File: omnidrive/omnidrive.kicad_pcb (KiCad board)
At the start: 2 copper layers, 76.2 x 27.9 mm, 73 parts, among them U1 TL072, U2 TL072

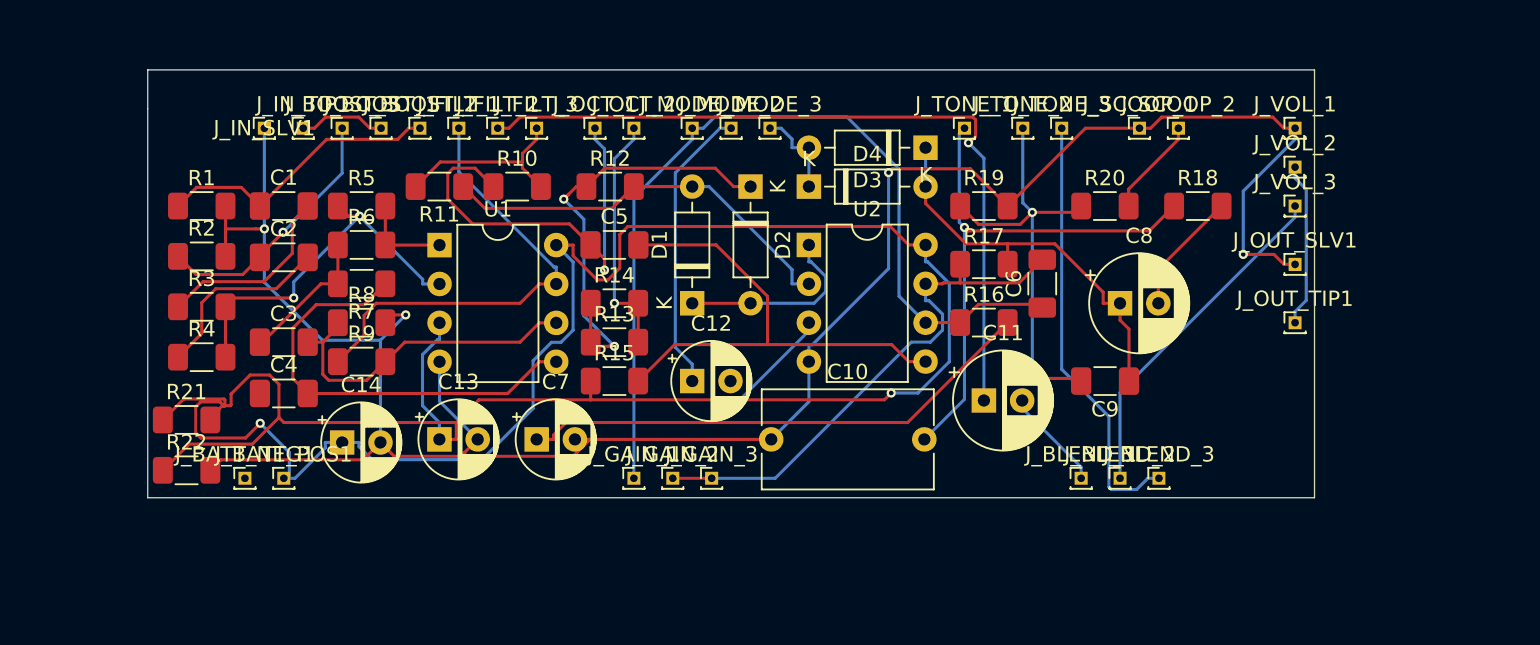
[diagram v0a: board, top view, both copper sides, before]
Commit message: stuff
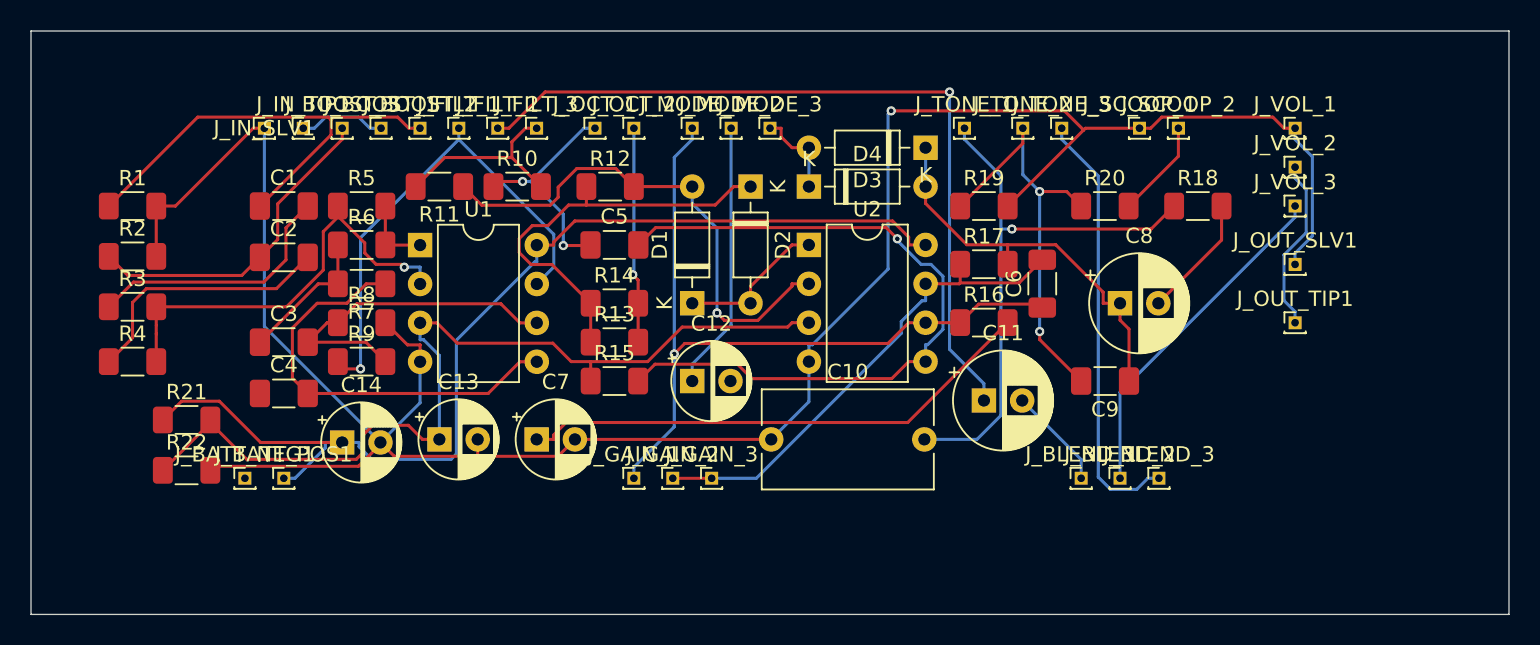
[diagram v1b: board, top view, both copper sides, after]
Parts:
- moved R4 4.53 mm to (24.4, 41.9)
- moved R1 4.52 mm to (24.4, 31.8)
- moved R2 4.52 mm to (24.4, 35.0)
- moved R3 4.52 mm to (24.4, 38.3)
- moved U1 1.27 mm to (43.2, 34.3)
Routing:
- net /Vb: track 91.4 -> 59.5 mm, vias 2 -> 0
- net Net-(U2B-+): track 33.2 -> 47.9 mm, vias 0 -> 1
- net Net-(J_OCT_1-Pin_1): track 29.0 -> 15.1 mm, vias 1 -> 2
- net Net-(J_BOOST_2-Pin_1): track 18.9 -> 30.7 mm
- net +9V: track 78.7 -> 69.5 mm, vias 1 -> 0
- net Net-(J_GAIN_1-Pin_1): track 58.6 -> 49.9 mm, vias 0 -> 1
- net GND: track 146.7 -> 155.0 mm, vias 4 -> 1
- net Net-(D1-A): track 26.9 -> 33.5 mm, vias 0 -> 1
- net Net-(C2-Pad2): track 12.3 -> 17.2 mm
- net Net-(D2-K): track 31.9 -> 27.2 mm, vias 2 -> 0
- net Net-(J_BOOST_3-Pin_1): track 17.0 -> 21.5 mm, vias 1 -> 0
- net Net-(C1-Pad2): track 12.4 -> 16.9 mm
- net Net-(U1A--): track 24.0 -> 28.6 mm, vias 2 -> 1
- net Net-(D1-K): track 12.6 -> 9.84 mm
- net Net-(J_FILT_1-Pin_1): track 30.0 -> 32.5 mm, vias 0 -> 1
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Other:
- board size 76.2 x 27.9 mm -> 96.5 x 38.1 mm
